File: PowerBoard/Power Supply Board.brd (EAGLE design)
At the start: 65.4 x 78.7 mm, 41 parts, among them IC3 LM2675

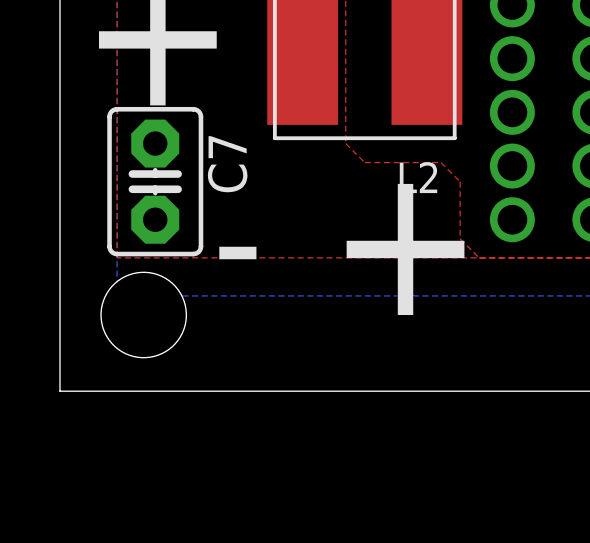
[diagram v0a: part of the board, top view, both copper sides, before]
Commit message: final changes for FAB
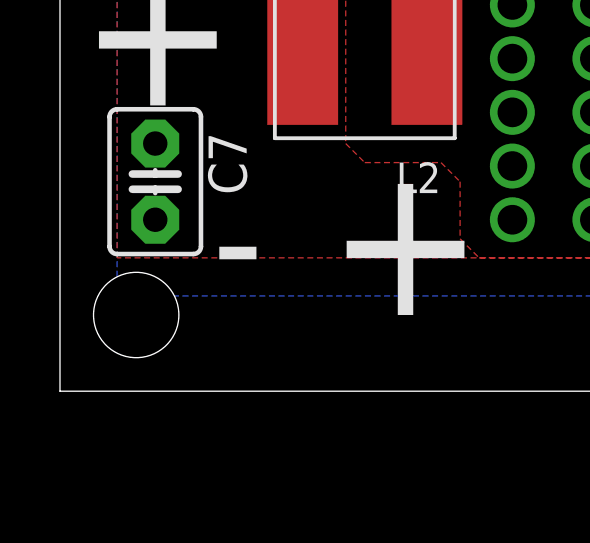
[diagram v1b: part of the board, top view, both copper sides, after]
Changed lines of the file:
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@@
 <hole x="62.865" y="76.2" drill="2.8448"/>
 <hole x="62.865" y="2.54" drill="2.8448"/>
-<hole x="2.79" y="2.54" drill="2.8448"/>
+<hole x="2.54" y="2.54" drill="2.8448"/>
 <hole x="2.54" y="39.37" drill="2.8448"/>
 <text x="5.08" y="3.175" size="3.81" layer="25">-</text>
